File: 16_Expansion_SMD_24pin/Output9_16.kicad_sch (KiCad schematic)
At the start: 28 parts, among them J10 String10, J11 String11, J12 String12, J13 String13, J14 String14, J15 String15, J16 String16, J9 String9, U2 74HC245

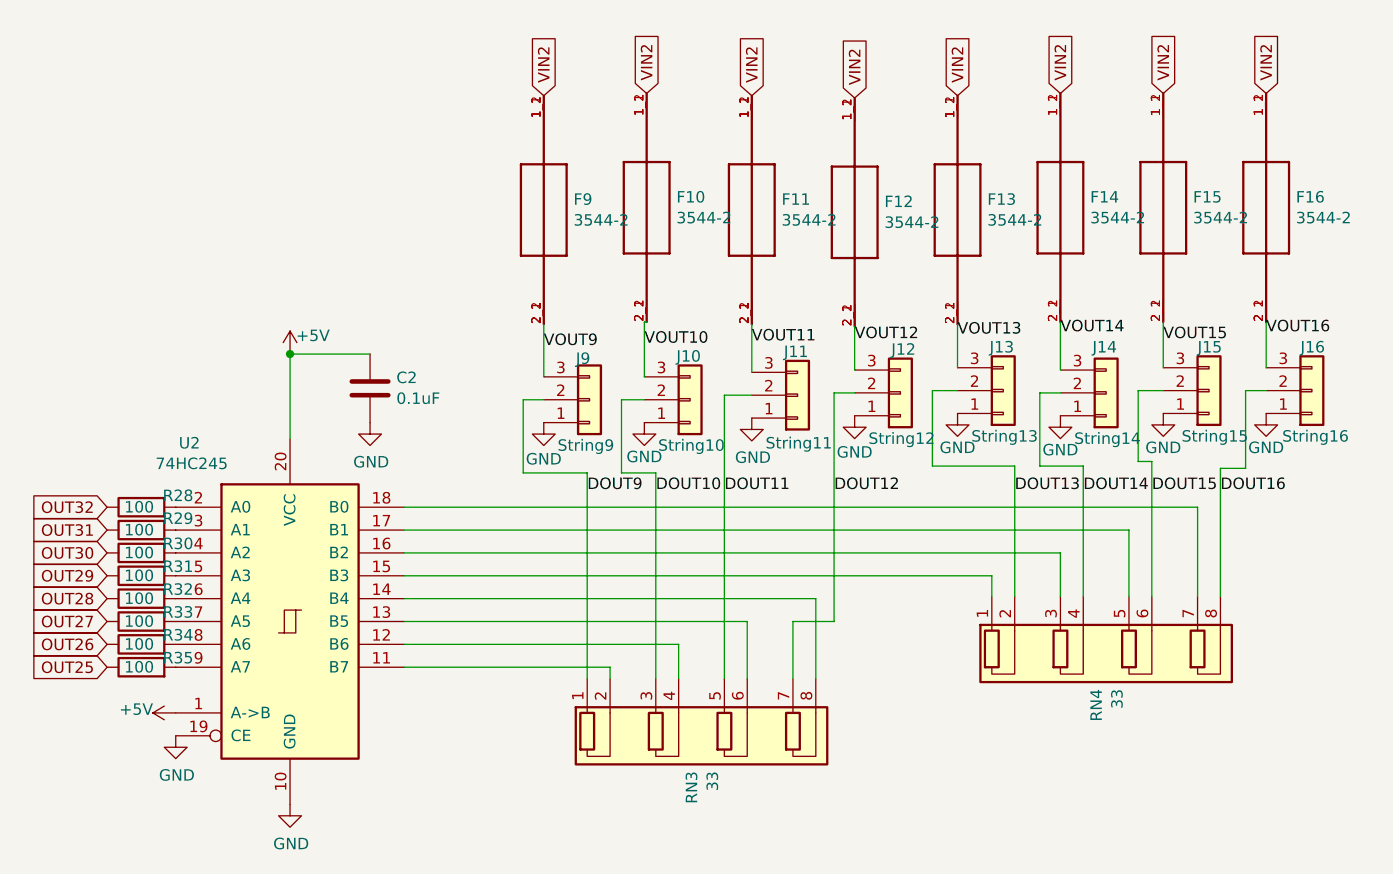
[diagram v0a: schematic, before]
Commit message: update 24pin
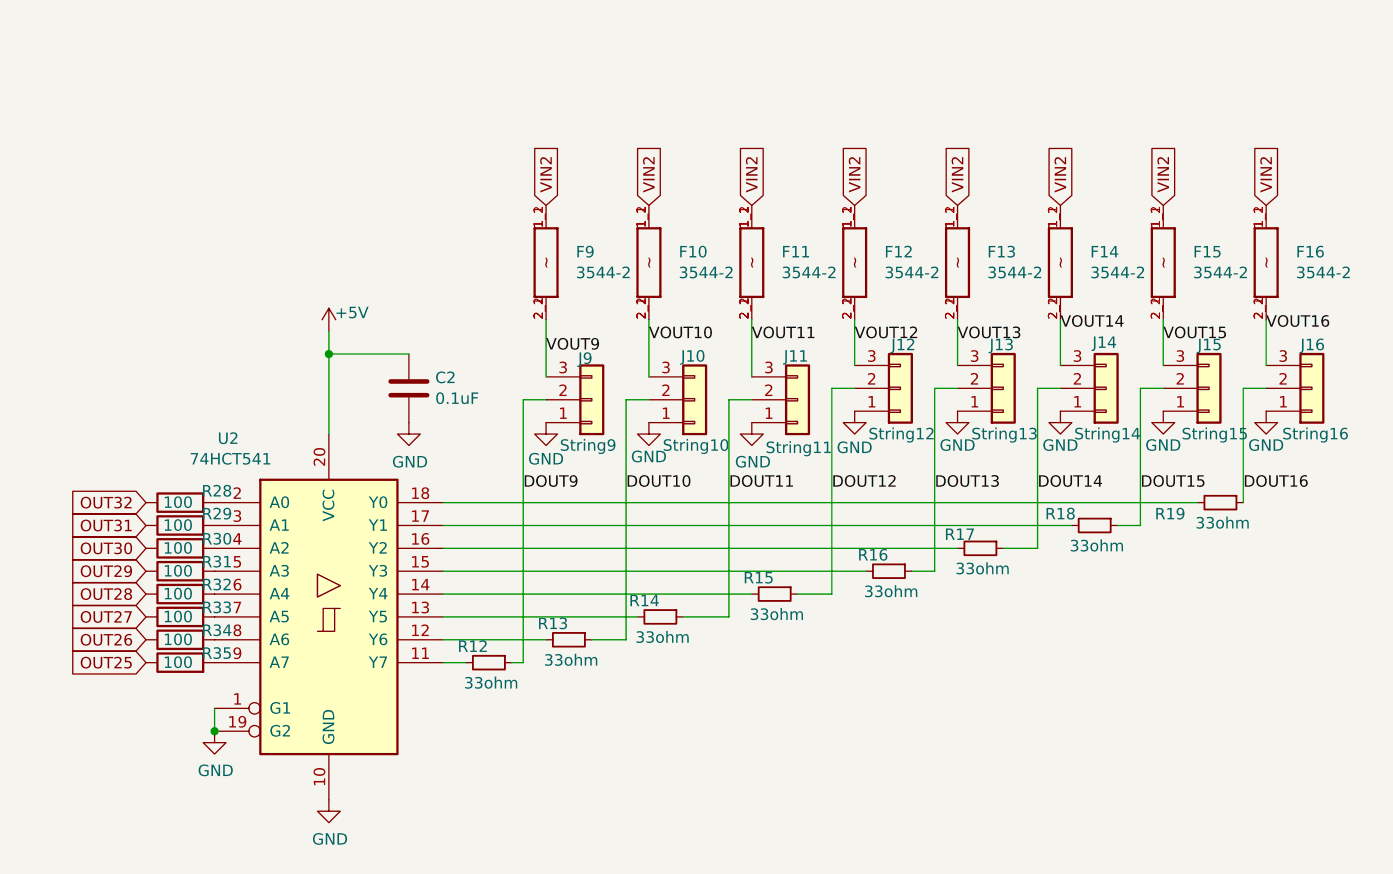
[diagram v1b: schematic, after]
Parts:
- removed RN3, RN4: 33, Resistor_THT:R_Array_SIP8, symbol PB_16-rescue:R_Pack04_SIP-Device
- added R12, R13, R14, R15, R16, R17, R18, R19: 33ohm, Resistor_SMD:R_0603_1608Metric, symbol Device:R_Small
- C2: footprint Capacitor_SMD:C_0805_2012Metric_Pad1.15x1.40mm_HandSolder -> Capacitor_SMD:C_0402_1005Metric
- F10, F11, F12, F13, F14, F15, F16, F9: footprint Keystone_Fuse:FUSE_3544-2 -> Scotts:FUSE_3544-2; symbol PB_16-rescue:3544-2-Keystone_Fuse -> Scotts:3544-2; LCSC (none) -> C492610
- J10, J11, J12, J13, J14, J15, J16, J9: footprint Connector_Phoenix_MC:PhoenixContact_MCV_1,5_3-G-3.5_1x03_P3.50mm_Vertical -> Scotts:PhoenixContact_MCV_3.81mm_3.5mm_1x03_Vertical
- R28, R29, R30, R31, R32, R33, R34, R35: footprint Resistor_SMD:R_0603_1608Metric_Pad0.98x0.95mm_HandSolder -> Resistor_SMD:R_0603_1608Metric
- U2: value 74HC245 -> 74HCT541; footprint Package_SO:SOIC-20W_7.5x12.8mm_P1.27mm -> Package_SO:TSSOP-20_4.4x6.5mm_P0.65mm; symbol 74xx:74HC245 -> 74xx:74HCT541; Digi-Key_PN 296-8279-1-ND -> (none); LCSC C5625 -> (none); MPN SN74HC245PWR -> (none)
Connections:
- net +5V: no longer U2.1 (A->B)
- net DOUT10: now also R13.1
- net DOUT11: now also R14.1
- net DOUT12: now also R15.1
- net DOUT13: now also R16.1
- net DOUT14: now also R17.1
- net DOUT15: now also R18.1
- net DOUT16: now also R19.1
- net DOUT9: now also R12.1
- net GND: now also U2.1 (G1)
- net at U2.15 (Y3): now also R16.2
- net at U2.16 (Y2): now also R17.2
- net at U2.17 (Y1): now also R18.2
- net at U2.18 (Y0): now also R19.2
- net at U2.11 (Y7): now also R12.2
- net at U2.12 (Y6): now also R13.2
- net at U2.13 (Y5): now also R14.2
- net at U2.14 (Y4): now also R15.2
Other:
- moved on the sheet: C2, F10, F11, F12, F13, F14, F15, F16, F9, J10, J11, J12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
